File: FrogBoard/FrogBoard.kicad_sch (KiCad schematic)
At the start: 44 parts, among them J1 Conn_01x10, J10 Conn_01x02, J11 Conn_01x01, J12 Conn_01x02, J13 Conn_01x01, J14 Conn_01x01, J15 Conn_01x01, J2 Conn_01x04, J3 USB_B_Micro, J4 Stickbox, J5 Conn_01x03_Socket, J6 Conn_01x02, J7 Conn_01x02, J8 Conn_01x01, J9 Conn_01x01, U1 STM32L432KBUx, U2 USBLC6-2P6, U3 MCP1700T-3302E, U4 BL1555

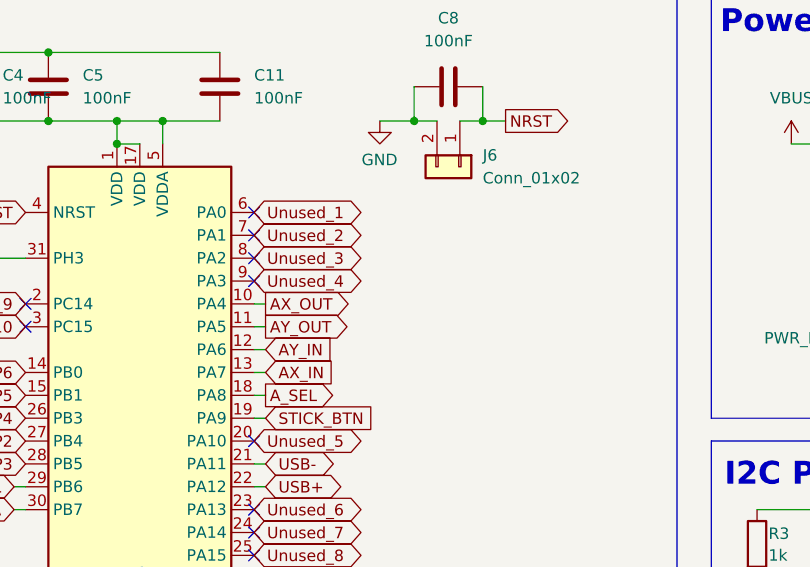
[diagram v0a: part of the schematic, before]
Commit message: Add LED
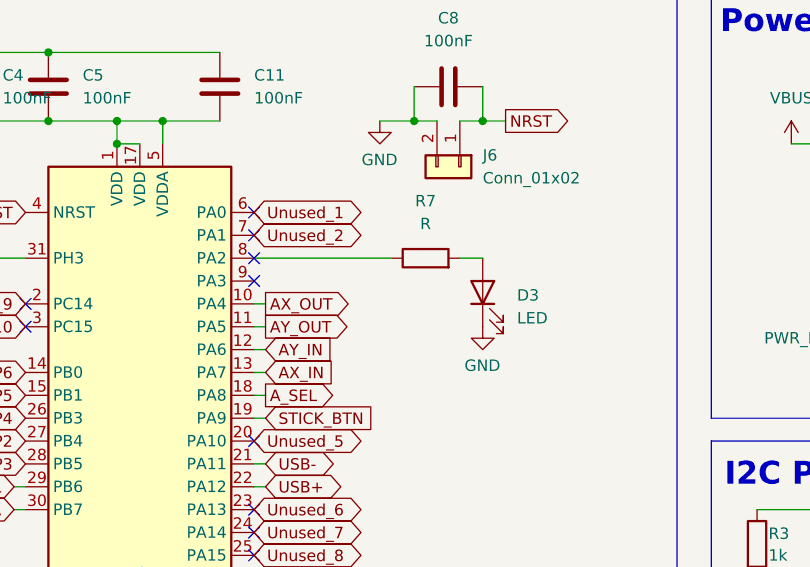
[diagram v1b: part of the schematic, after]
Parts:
- added D3: LED, LED_SMD:LED_0603_1608Metric, symbol Device:LED
- added R7: R, Resistor_SMD:R_0603_1608Metric, symbol Device:R
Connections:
- net GND: now also D3.1 (K)
- net Unused_3: no longer U1.8 (PA2)
- net Unused_4: no longer U1.9 (PA3)
- new net: R7.1, U1.8 (PA2)
- new net: D3.2 (A), R7.2
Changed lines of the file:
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@@
 	(wire
 		(pts
+			(xy 109.22 45.72) (xy 111.76 45.72)
+		)
+		(stroke
+			(width 0)
+			(type default)
+		)
+	)
+	(wire
+		(pts
 			(xy 87.63 50.8) (xy 86.36 50.8)
 		)
@@
 	(wire
 		(pts
+			(xy 86.36 45.72) (xy 101.6 45.72)
+		)
+		(stroke
+			(width 0)
+			(type default)
+		)
+	)
+	(wire
+		(pts
 			(xy 148.59 127) (xy 149.86 127)
 		)
@@
 		)
 	)
-	(global_label "Unused_3"
-		(shape bidirectional)
-		(at 86.36 45.72 0)
-		(fields_autoplaced yes)
-		(effects
-			(font
-				(size 1.27 1.27)
-			)
-			(justify left)
-		)
-		(property "Intersheetrefs" "${INTERSHEET_REFS}"
-			(at 99.5278 45.72 0)
-			(effects
-				(font
-					(size 1.27 1.27)
-				)
-				(justify left)
-				(hide yes)
-			)
-		)
-	)
 	(global_label "AX_MUX_OUT"
 		(shape input)
@@
 		)
 	)
-	(global_label "Unused_4"
-		(shape bidirectional)
-		(at 86.36 48.26 0)
-		(fields_autoplaced yes)
-		(effects
-			(font
-				(size 1.27 1.27)
-			)
-			(justify left)
-		)
-		(property "Intersheetrefs" "${INTERSHEET_REFS}"
-			(at 99.5278 48.26 0)
-			(effects
-				(font
-					(size 1.27 1.27)
-				)
-				(justify left)
-				(hide yes)
-			)
-		)
-	)
 	(global_label "Unused_5"
 		(shape bidirectional)
@@
 	)
 	(symbol
+		(lib_id "Device:R")
+		(at 105.41 45.72 90)
+		(unit 1)
+		(exclude_from_sim no)
+		(in_bom yes)
+		(on_board yes)
+		(dnp no)
+		(fields_autoplaced yes)
+		(property "Reference" "R7"
+			(at 105.41 39.37 90)
+			(effects
+				(font
+					(size 1.27 1.27)
+				)
+			)
+		)
+		(property "Value" "R"
+			(at 105.41 41.91 90)
+			(effects
+				(font
+					(size 1.27 1.27)
+				)
+			)
+		)
+		(property "Footprint" "Resistor_SMD:R_0603_1608Metric"
+			(at 105.41 47.498 90)
+			(effects
+				(font
+					(size 1.27 1.27)
+				)
+				(hide yes)
+			)
+		)
+		(property "Datasheet" "~"
+			(at 105.41 45.72 0)
+			(effects
+				(font
+					(size 1.27 1.27)
+				)
+				(hide yes)
+			)
+		)
+		(property "Description" "Resistor"
+			(at 105.41 45.72 0)
+			(effects
+				(font
+					(size 1.27 1.27)
+				)
+				(hide yes)
+			)
+		)
+		(pin "1"
+		)
+		(pin "2"
+		)
+		(instances
+			(project ""
+				(path "/70a1c624-543f-486d-b6f1-90effc8a6c8b"
+					(reference "R7")
+					(unit 1)
+				)
+			)
+		)
+	)
+	(symbol
 		(lib_id "power:+3.3V")
 		(at 19.05 30.48 180)
@@
 	)
 	(symbol
+		(lib_id "power:GND")
+		(at 111.76 53.34 0)
+		(unit 1)
+		(exclude_from_sim no)
+		(in_bom yes)
+		(on_board yes)
+		(dnp no)
+		(property "Reference" "#PWR013"
+			(at 111.76 59.69 0)
+			(effects
+				(font
+					(size 1.27 1.27)
+				)
+				(hide yes)
+			)
+		)
+		(property "Value" "GND"
+			(at 109.728 57.658 0)
+			(effects
+				(font
+					(size 1.27 1.27)
+				)
+				(justify left)
+			)
+		)
+		(property "Footprint" ""
+			(at 111.76 53.34 0)
+			(effects
+				(font
+					(size 1.27 1.27)
+				)
+				(hide yes)
+			)
+		)
+		(property "Datasheet" ""
+			(at 111.76 53.34 0)
+			(effects
+				(font
+					(size 1.27 1.27)
+				)
+				(hide yes)
+			)
+		)
+		(property "Description" "Power symbol creates a global label with name \"GND\" , ground"
+			(at 111.76 53.34 0)
+			(effects
+				(font
+					(size 1.27 1.27)
+				)
+				(hide yes)
+			)
+		)
+		(pin "1"
+		)
+		(instances
+			(project "FrogBoard"
+				(path "/70a1c624-543f-486d-b6f1-90effc8a6c8b"
+					(reference "#PWR013")
+					(unit 1)
+				)
+			)
+		)
+	)
+	(symbol
 		(lib_id "Device:R")
 		(at 153.67 77.47 0)
@@
 					(unit 1)
 				)
+			)
+		)
+	)
+	(symbol
+		(lib_id "Device:LED")
+		(at 111.76 49.53 90)
+		(unit 1)
+		(exclude_from_sim no)
+		(in_bom yes)
+		(on_board yes)
+		(dnp no)
+		(fields_autoplaced yes)
+		(property "Reference" "D3"
+			(at 115.57 49.8474 90)
+			(effects
+				(font
+					(size 1.27 1.27)
+				)
+				(justify right)
+			)
+		)
+		(property "Value" "LED"
+			(at 115.57 52.3874 90)
+			(effects
+				(font
+					(size 1.27 1.27)
+				)
+				(justify right)
+			)
+		)
+		(property "Footprint" "LED_SMD:LED_0603_1608Metric"
+			(at 111.76 49.53 0)
+			(effects
+				(font
+					(size 1.27 1.27)
+				)
+				(hide yes)
+			)
+		)
+		(property "Datasheet" "~"
+			(at 111.76 49.53 0)
+			(effects
+				(font
+					(size 1.27 1.27)
+				)
+				(hide yes)
+			)
+		)
+		(property "Description" "Light emitting diode"
+			(at 111.76 49.53 0)
+			(effects
+				(font
+					(size 1.27 1.27)
+				)
+				(hide yes)
+			)
+		)
+		(property "Sim.Pins" "1=K 2=A"
+			(at 111.76 49.53 0)
+			(effects
+				(font
+					(size 1.27 1.27)
+				)
+				(hide yes)
+			)
+		)
+		(pin "1"
+		)
+		(pin "2"
+		)
+		(instances
+			(project ""
+				(path "/70a1c624-543f-486d-b6f1-90effc8a6c8b"
+					(reference "D3")
+					(unit 1)
+				)
